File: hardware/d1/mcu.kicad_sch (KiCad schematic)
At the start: 26 parts, among them J3 SWD, J4 UART, Q3 DMG1012T-7, SW1 SSSS811101, U2 STM32G0B1VCT6

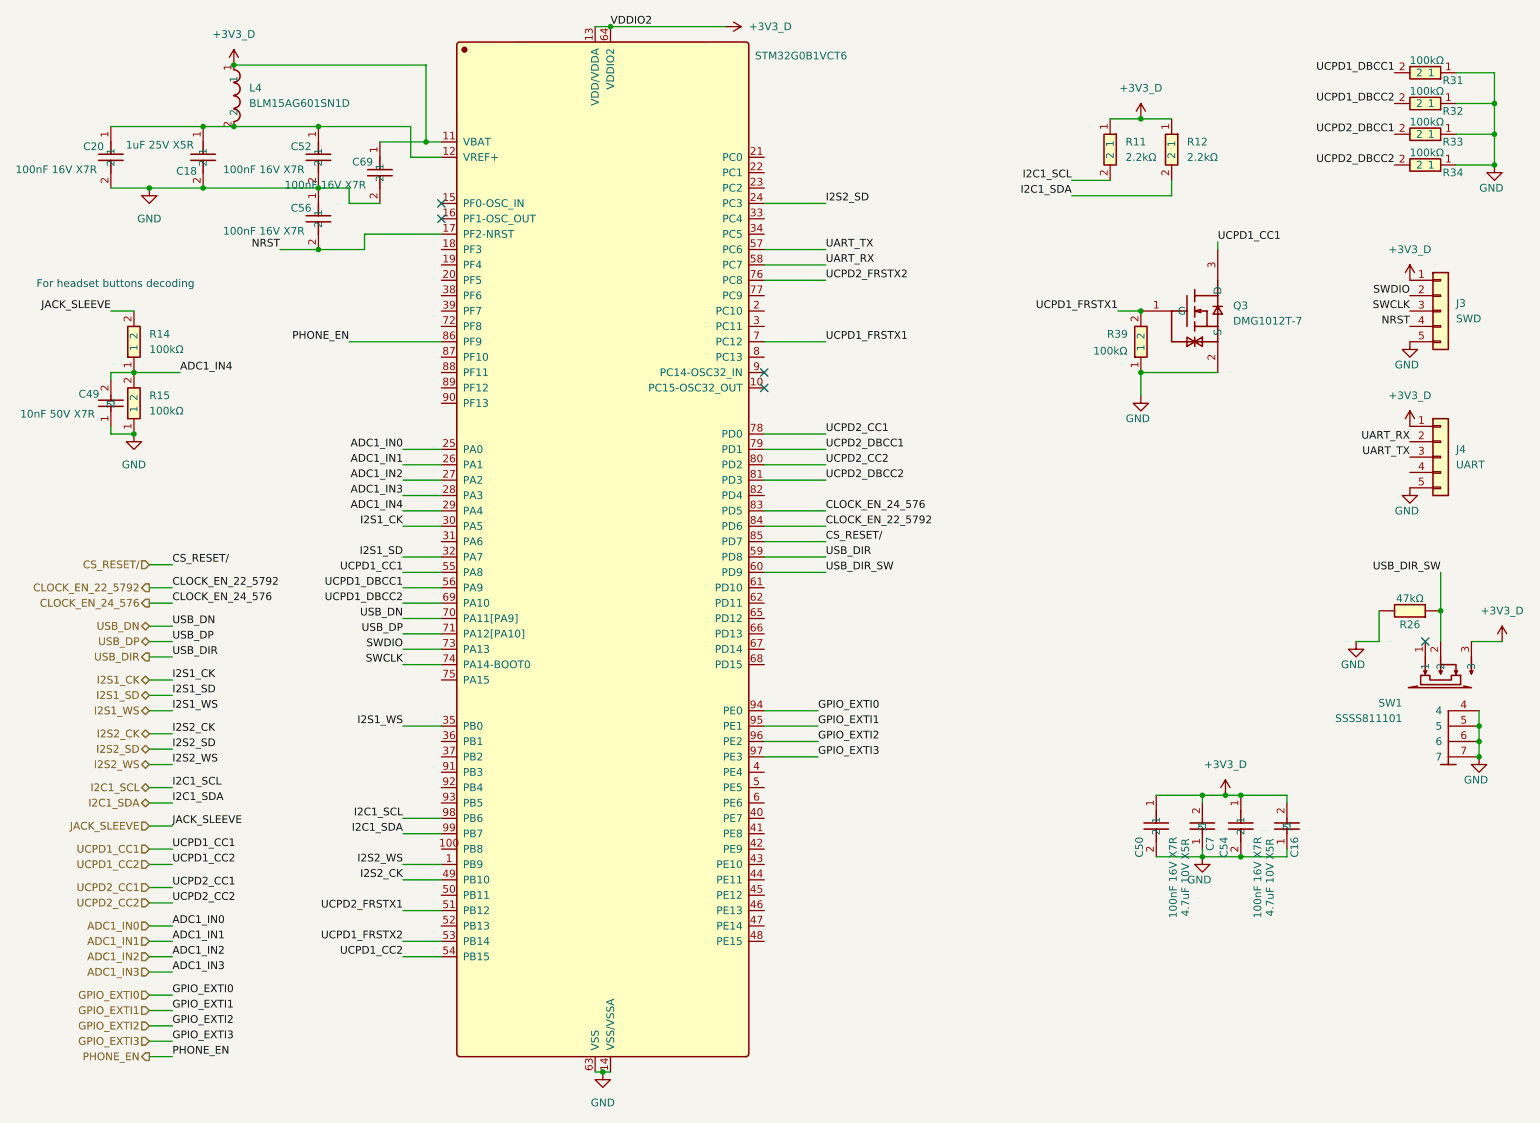
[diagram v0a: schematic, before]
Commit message: Replace parts
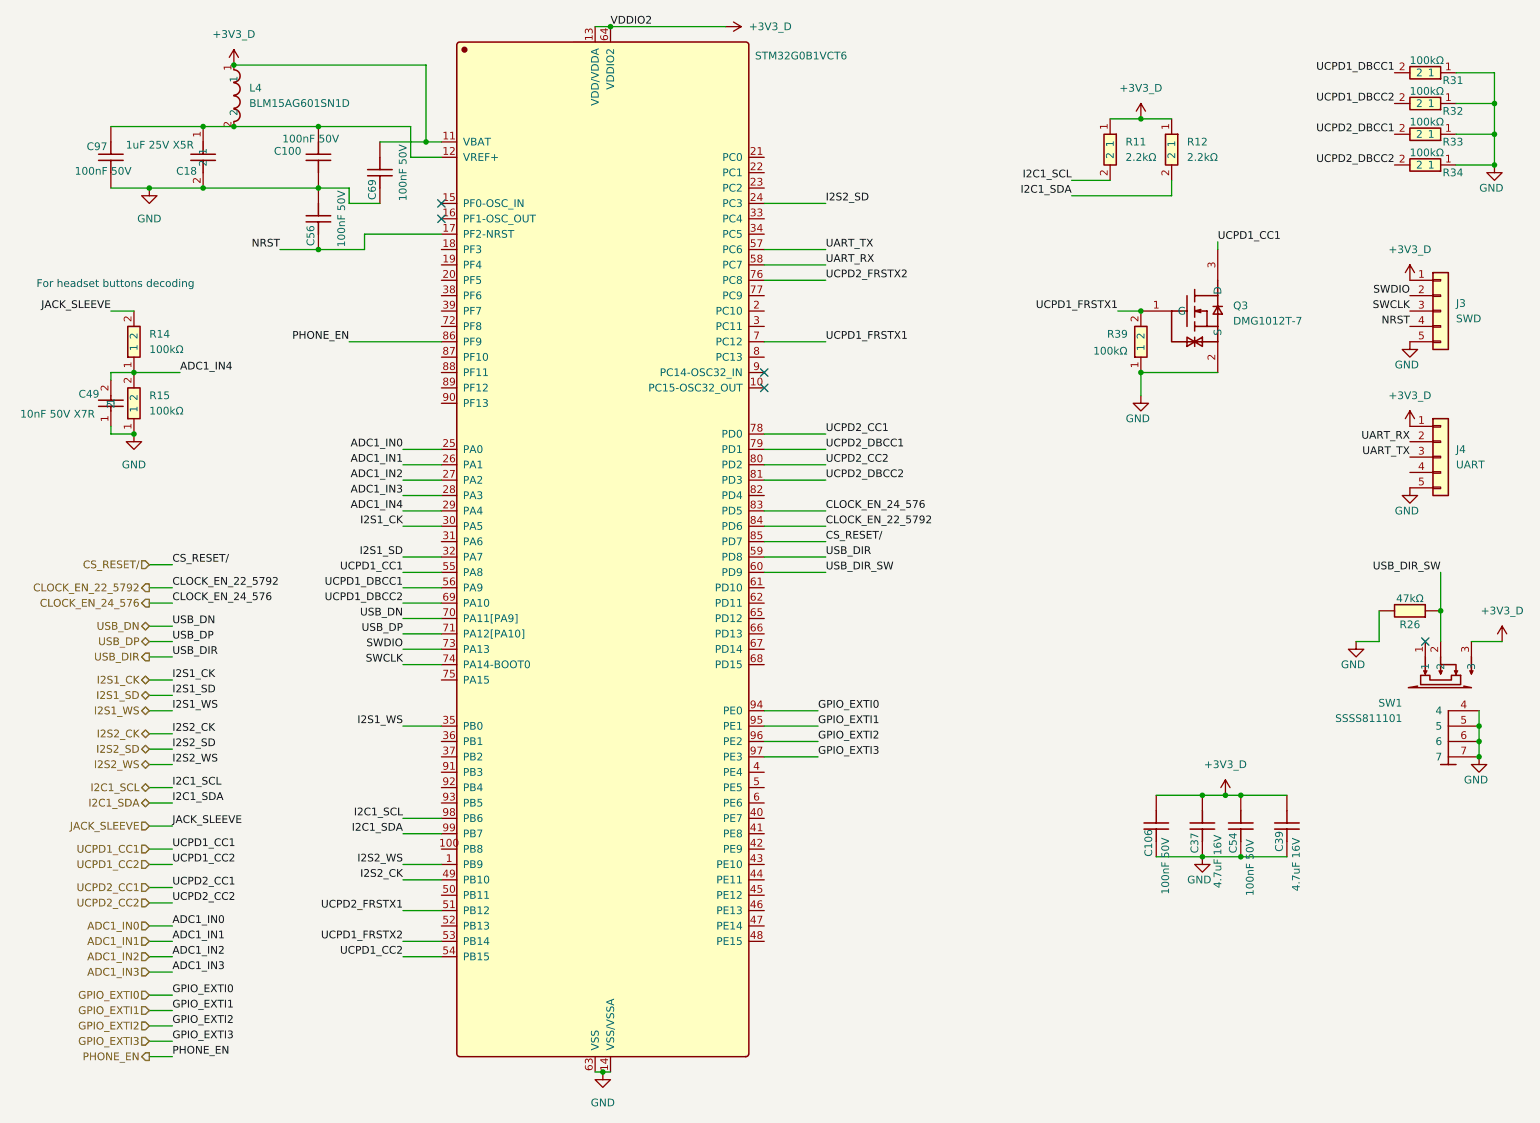
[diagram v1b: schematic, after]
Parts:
- removed C16, C7: 4.7uF 10V X5R, Capacitor_SMD:C_0603_1608Metric, symbol JLCImport:CL10A475KP8NNNC
- removed C20, C50, C52, C54, C56, C69: 100nF 16V X7R, JLCImport:CL05B104KO5NNNC, symbol JLCImport:CL05B104KO5NNNC
- added C100, C106, C54, C56, C69, C97: 100nF 50V, Capacitor_SMD:C_0402_1005Metric, symbol JLCImport:CL05B104KB54PNC
- added C37, C39: 4.7uF 16V, Capacitor_SMD:C_0603_1608Metric, symbol JLCImport:CL10A475KO8NNNC
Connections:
- net +3V3_D: now also C106.2, C37.2, C39.2, C54.2, C69.2
- net GND: now also C100.1, C106.1, C37.1, C39.1, C54.1, C56.2, C69.1, C97.1
- net NRST: now also C56.1
- net at C18.1, L4.2, U2.12 (VREF+): now also C100.2, C97.2
